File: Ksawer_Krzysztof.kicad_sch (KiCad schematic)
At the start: 35 parts, among them K1 1461103-1, K2 1461103-1, Q1 BC547, Q2 MMBT3904, Q3 MMBT3904, U1 DHT11, U2 ESP-12E, U3 NHD-C0220BIZ, U4 LTV-844, U5 STM32F038K6Ux

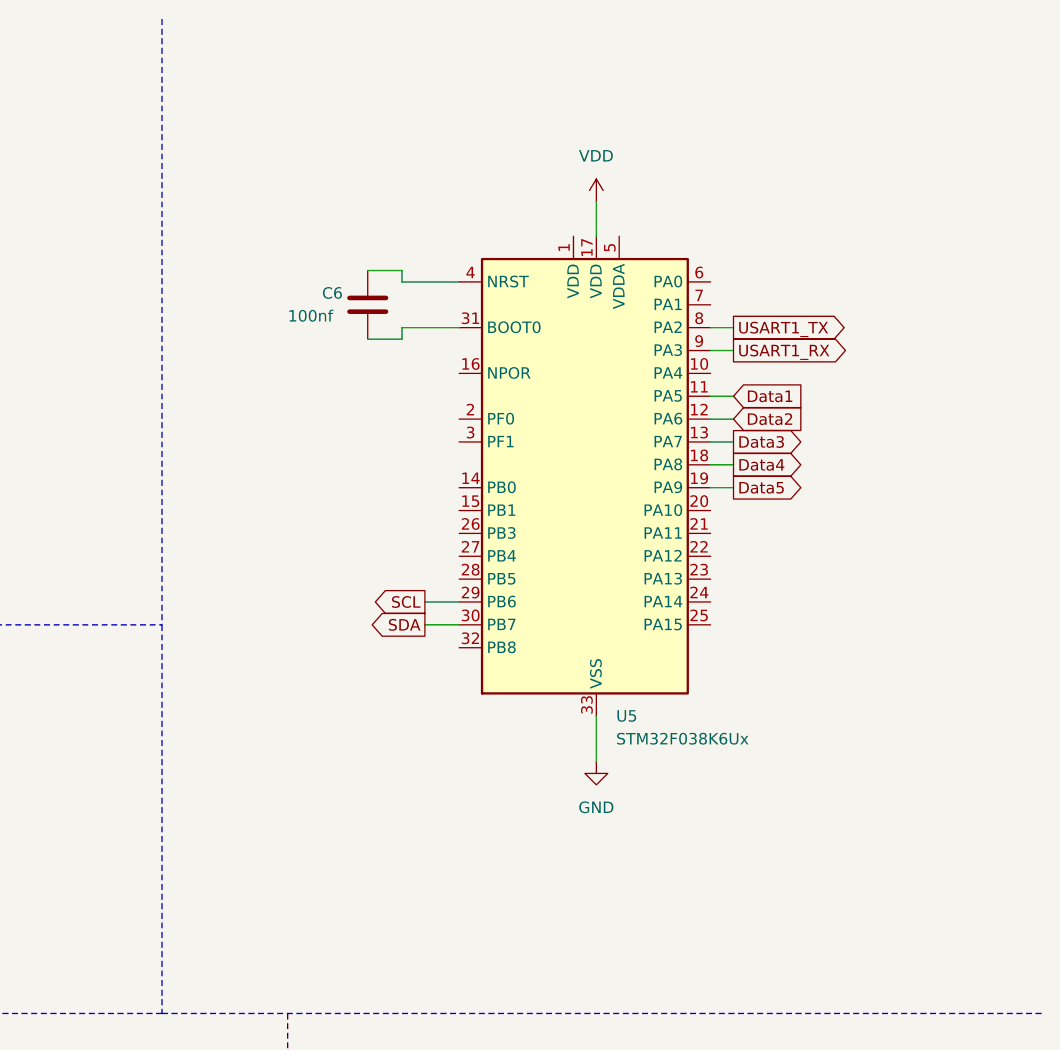
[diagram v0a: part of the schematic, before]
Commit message: zmiany2
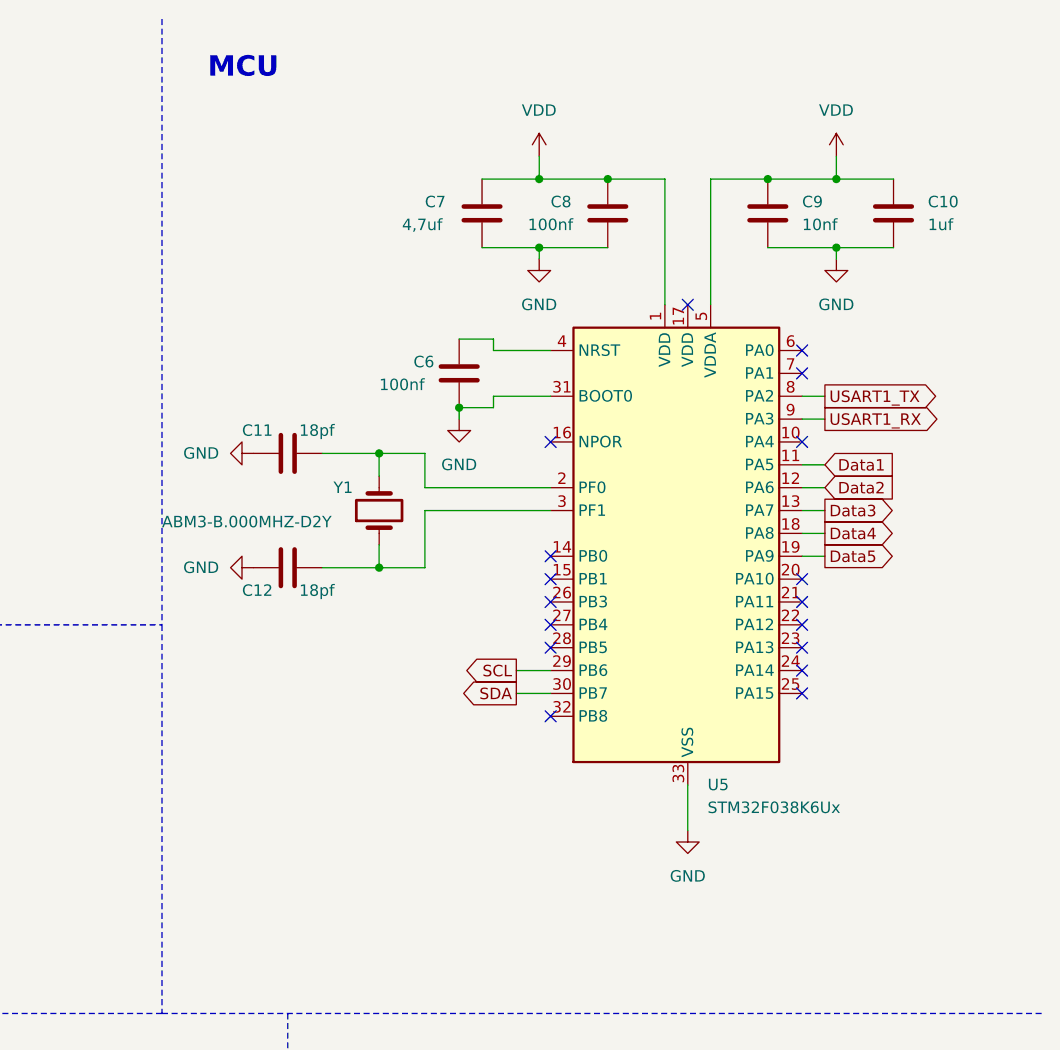
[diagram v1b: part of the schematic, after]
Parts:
- added C10: 1uf, symbol Device:C
- added C11, C12: 18pf, symbol Device:C
- added C7: 4,7uf, symbol Device:C
- added C8: 100nf, symbol Device:C
- added C9: 10nf, symbol Device:C
- added Y1: ABM3-B.000MHZ-D2Y, symbol Device:Crystal
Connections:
- net GND: now also C6.2, U5.31 (BOOT0), C10.2, C11.2, C12.2, C7.2, C8.2, C9.2
- net VDD: now also U5.1 (VDD), U5.5 (VDDA), C10.1, C7.1, C8.1, C9.1; no longer U5.17 (VDD)
- net at U5.2 (PF0): now also C11.1, Y1.2
- net at U5.3 (PF1): now also C12.1, Y1.1
- no-connect marks 13 -> 30
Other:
- note added: "MCU"
- moved on the sheet: C6, U5
